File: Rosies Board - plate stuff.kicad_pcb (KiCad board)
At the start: 2 copper layers, 216.7 x 83.3 mm, 91 parts

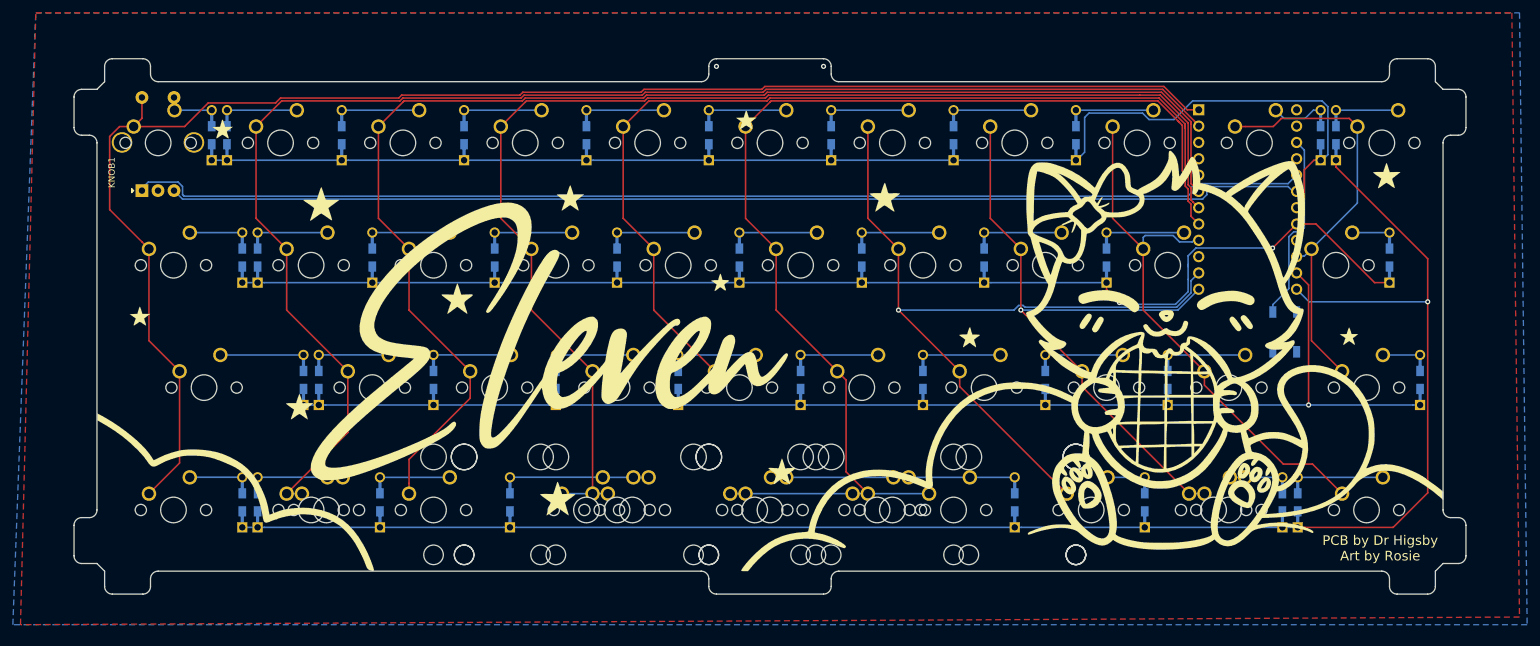
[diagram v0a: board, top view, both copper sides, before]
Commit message: eleven with tabs update
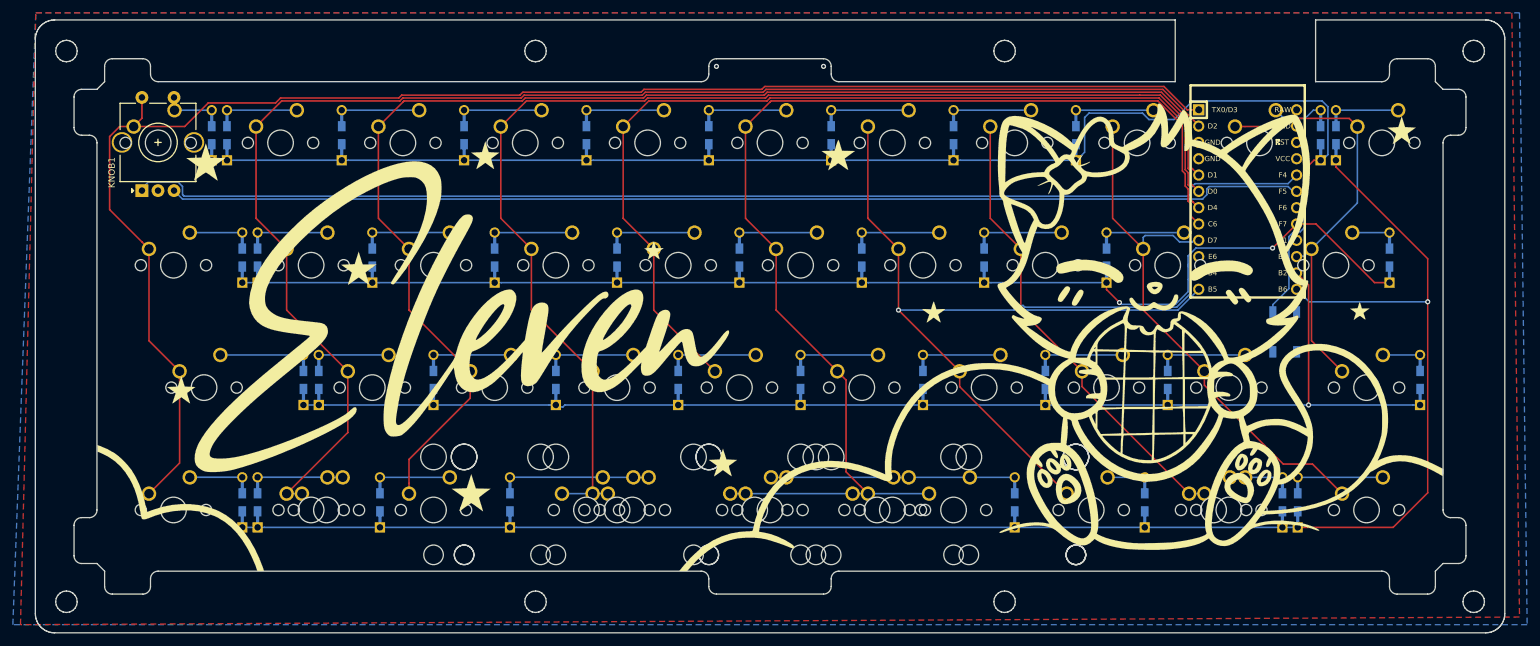
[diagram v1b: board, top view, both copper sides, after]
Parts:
- removed the G*** at (133.4, 54.8) (x2)
- added G***: LOGO, Eleven:eleven art 1, B.Cu at (133.4, 54.8)
- added G***: LOGO, Eleven:eleven art 1, F.Cu at (133.4, 54.8)
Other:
- board size 216.7 x 83.3 mm -> 228.8 x 95.4 mm
- board text added: "Eleven by: Rosie"
- board text removed: "PCB by Dr Higsby Art by Rosie"
